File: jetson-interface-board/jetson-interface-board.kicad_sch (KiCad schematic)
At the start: 32 parts, among them J1 Conn_01x04, J2 Conn_01x04, J3 USB_C_Receptacle_USB2.0, J4 Conn_01x04, J5 Conn_01x18, U1 MCP2562-E-MF, U2 FT234XD, U3 XC8111AA01MR-G

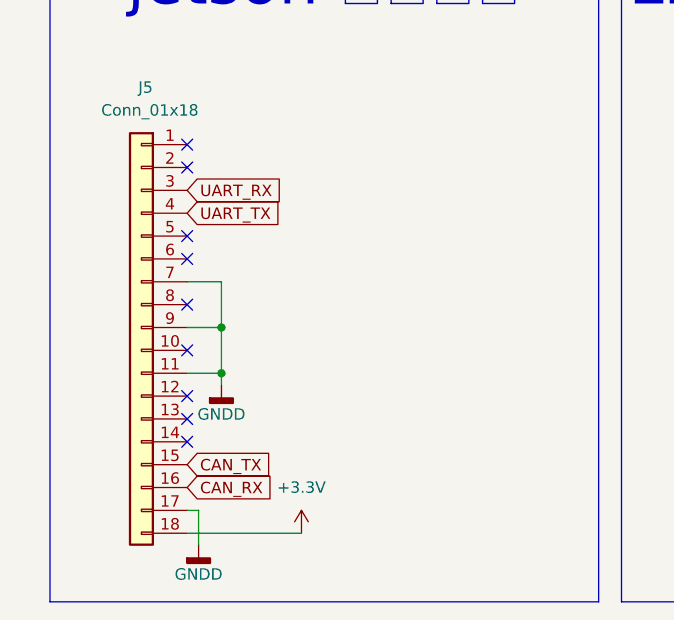
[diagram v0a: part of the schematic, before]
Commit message: fix:[WIP]pin header
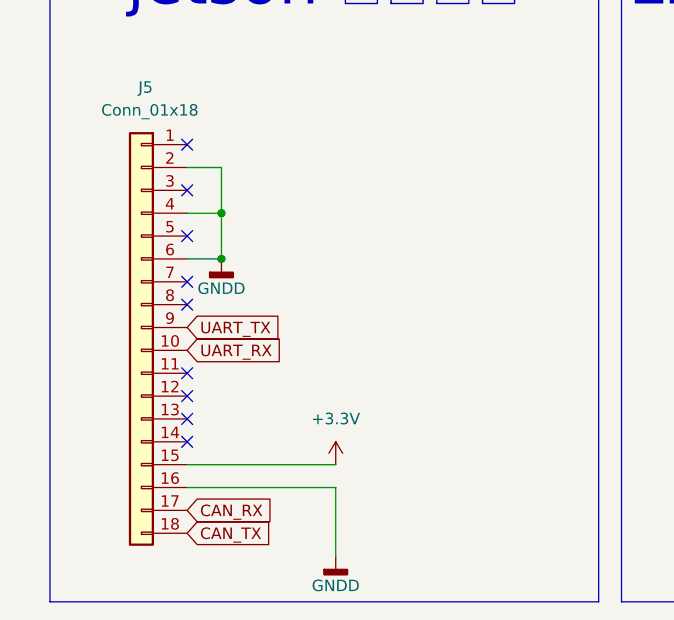
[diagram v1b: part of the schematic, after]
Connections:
- net +3.3V: now also J5.15 (Pin_15); no longer J5.18 (Pin_18)
- net CAN_RX: now also J5.17 (Pin_17); no longer J5.16 (Pin_16)
- net CAN_TX: now also J5.18 (Pin_18); no longer J5.15 (Pin_15)
- net GNDD: now also J5.16 (Pin_16), J5.2 (Pin_2), J5.4 (Pin_4), J5.6 (Pin_6); no longer J5.11 (Pin_11), J5.17 (Pin_17), J5.7 (Pin_7), J5.9 (Pin_9)
- net UART_RX: now also J5.10 (Pin_10); no longer J5.3 (Pin_3)
- net UART_TX: now also J5.9 (Pin_9); no longer J5.4 (Pin_4)
